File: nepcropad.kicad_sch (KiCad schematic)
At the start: 34 parts, among them SW1 SW_Push, U1 ATmega32U4-A, Y1 16MHz

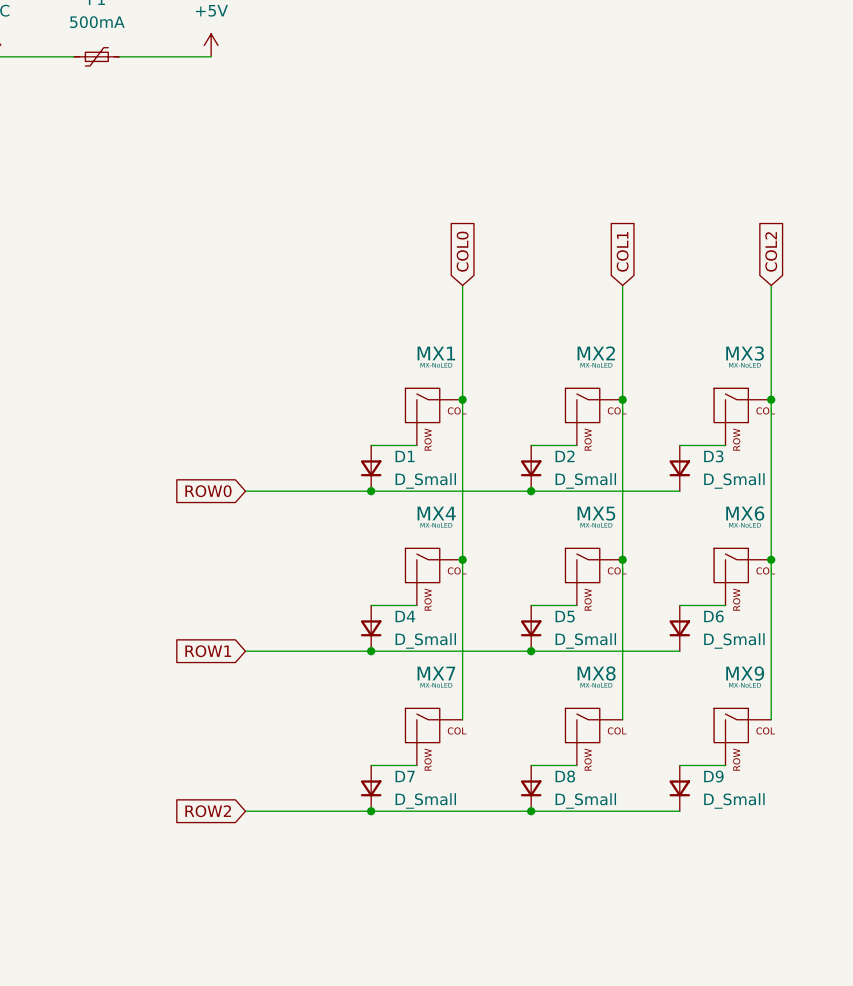
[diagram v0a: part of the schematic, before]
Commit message: PCB Layout
did the pcb layout
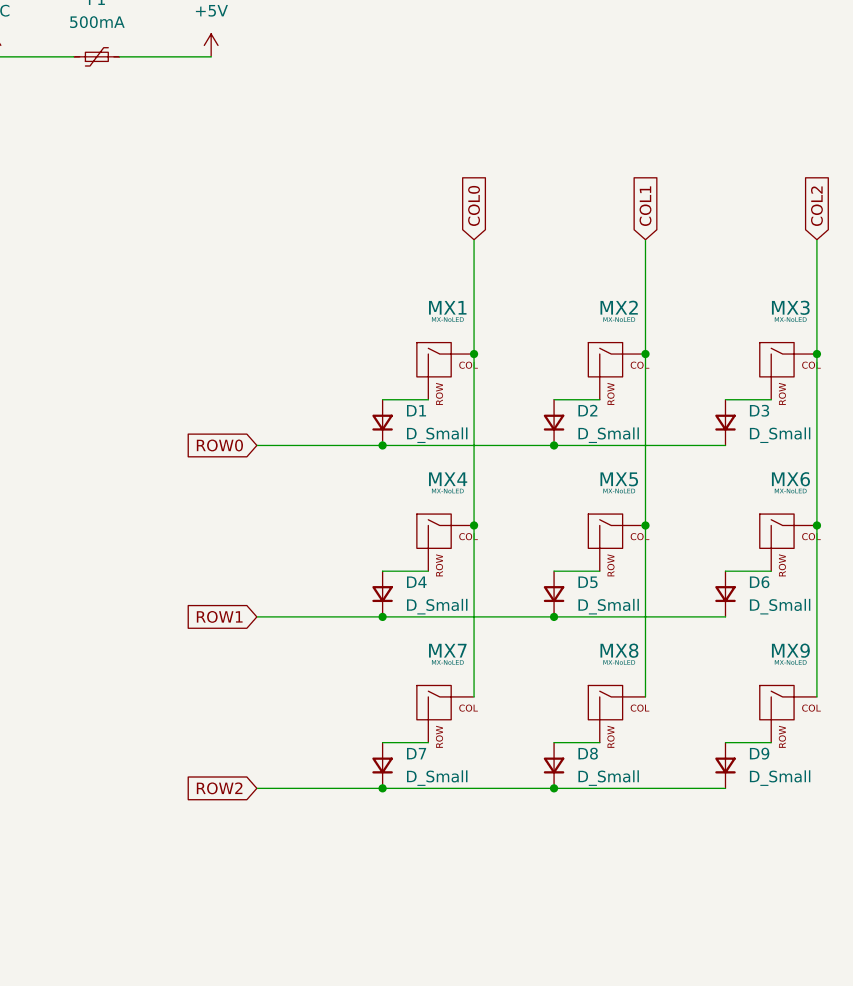
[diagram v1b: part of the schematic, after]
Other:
- moved on the sheet: D1, D2, D3, D4, D5, D6, D7, D8, D9, MX1, MX2, MX3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

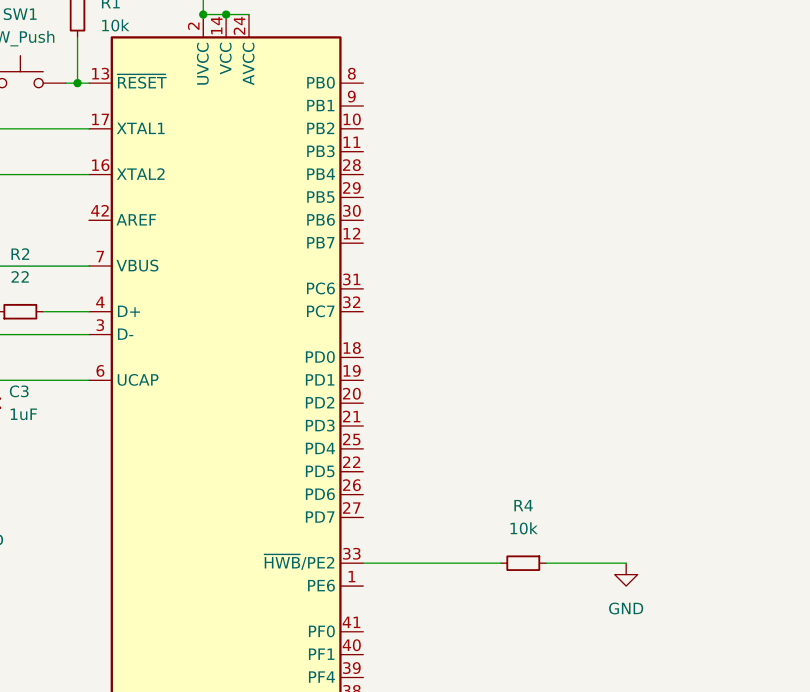
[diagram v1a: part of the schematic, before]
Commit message: Finished routing
I think atleast.
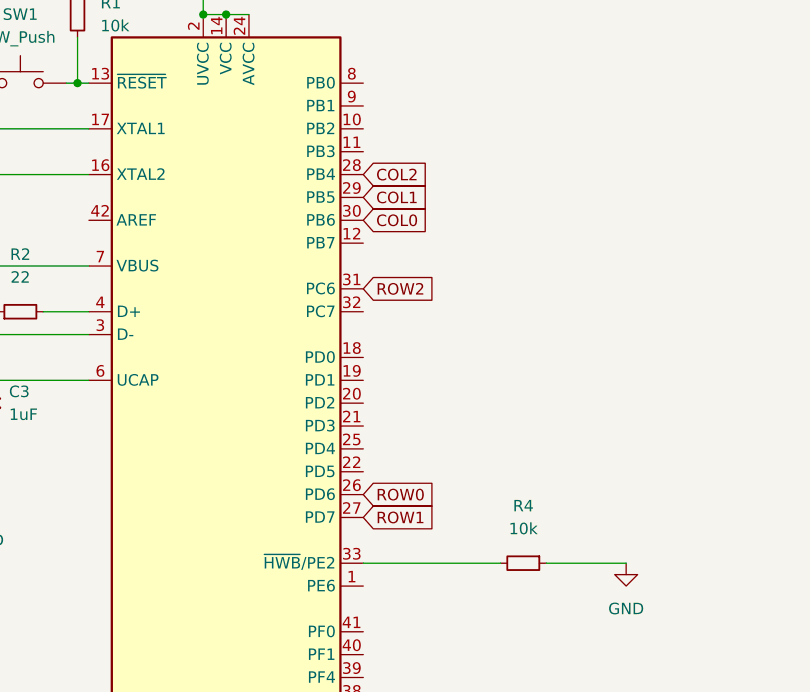
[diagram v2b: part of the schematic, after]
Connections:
- net COL0: now also U1.30 (PB6)
- net COL1: now also U1.29 (PB5)
- net COL2: now also U1.28 (PB4)
- net ROW0: now also U1.26 (PD6)
- net ROW1: now also U1.27 (PD7)
- net ROW2: now also U1.31 (PC6)
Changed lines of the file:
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@@
+    )
+  )
+  (global_label "ROW1" (shape input) (at 104.14 119.38 0) (fields_autoplaced)
+    (effects (font (size 1.27 1.27)) (justify left))
+    (property "Intersheet References" "${INTERSHEET_REFS}" (id 0) (at 111.8145 119.3006 0)
+      (effects (font (size 1.27 1.27)) (justify left) hide)
+    )
+  )
+  (global_label "ROW2" (shape input) (at 104.14 93.98 0) (fields_autoplaced)
+    (effects (font (size 1.27 1.27)) (justify left))
+    (property "Intersheet References" "${INTERSHEET_REFS}" (id 0) (at 111.8145 93.9006 0)
+      (effects (font (size 1.27 1.27)) (justify left) hide)
     )
   )
@@
     (effects (font (size 1.27 1.27)) (justify left))
     (property "Intersheet References" "${INTERSHEET_REFS}" (id 0) (at 136.0655 35.6394 0)
+      (effects (font (size 1.27 1.27)) (justify left) hide)
+    )
+  )
+  (global_label "ROW0" (shape input) (at 104.14 116.84 0) (fields_autoplaced)
+    (effects (font (size 1.27 1.27)) (justify left))
+    (property "Intersheet References" "${INTERSHEET_REFS}" (id 0) (at 111.8145 116.7606 0)
       (effects (font (size 1.27 1.27)) (justify left) hide)
     )
@@
     )
   )
+  (global_label "COL2" (shape input) (at 104.14 81.28 0) (fields_autoplaced)
+    (effects (font (size 1.27 1.27)) (justify left))
+    (property "Intersheet References" "${INTERSHEET_REFS}" (id 0) (at 111.3912 81.2006 0)
+      (effects (font (size 1.27 1.27)) (justify left) hide)
+    )
+  )
+  (global_label "COL1" (shape input) (at 104.14 83.82 0) (fields_autoplaced)
+    (effects (font (size 1.27 1.27)) (justify left))
+    (property "Intersheet References" "${INTERSHEET_REFS}" (id 0) (at 111.3912 83.7406 0)
+      (effects (font (size 1.27 1.27)) (justify left) hide)
+    )
+  )
   (global_label "ROW2" (shape input) (at 166.37 114.3 180) (fields_autoplaced)
     (effects (font (size 1.27 1.27)) (justify right))
@@
       (effects (font (size 1.27 1.27)) (justify left) hide)
     )
+  )
+  (global_label "COL0" (shape input) (at 104.14 86.36 0) (fields_autoplaced)
+    (effects (font (size 1.27 1.27)) (justify left))
+    (property "Intersheet References" "${INTERSHEET_REFS}" (id 0) (at 111.3912 86.2806 0)
+      (effects (font (size 1.27 1.27)) (justify left) hide)
+    )

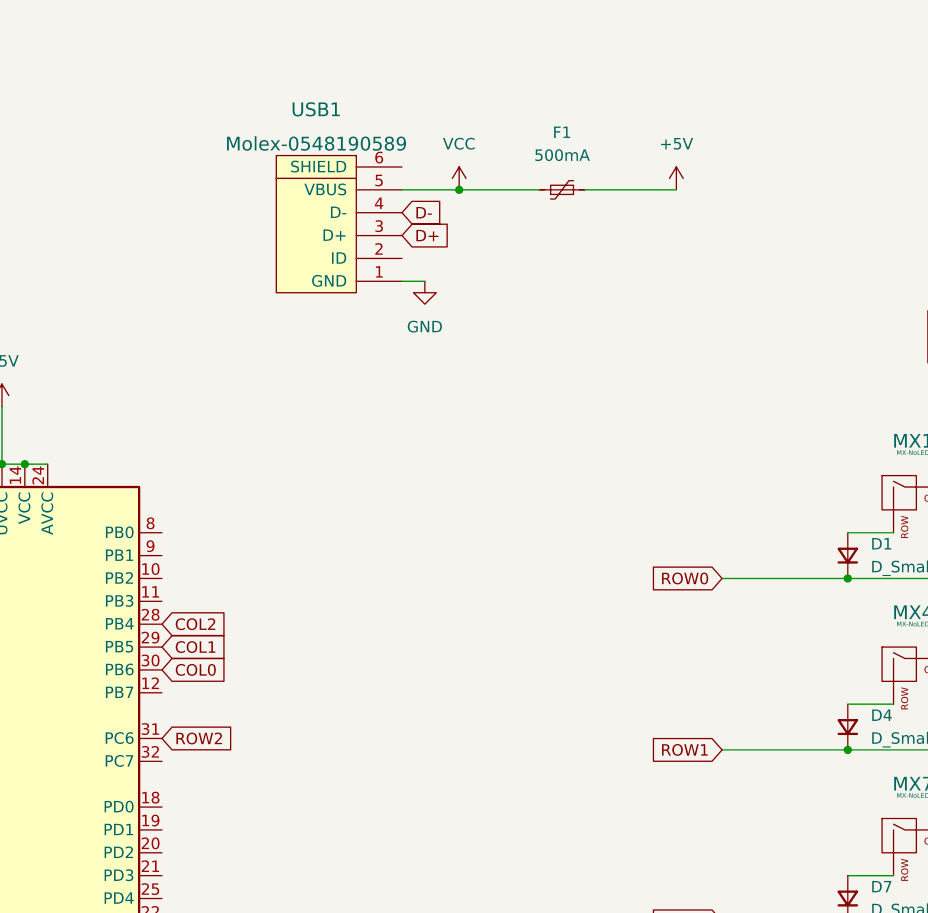
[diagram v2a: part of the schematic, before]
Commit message: minimize pcb
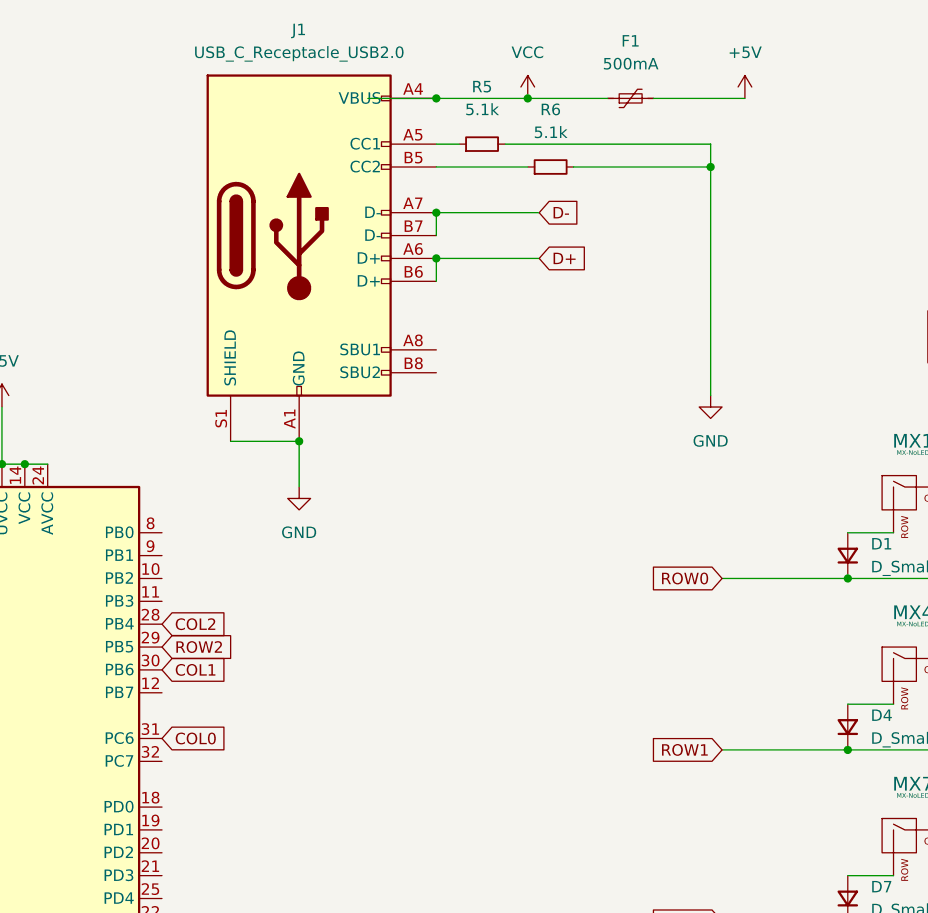
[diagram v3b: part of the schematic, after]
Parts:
- removed USB1: Molex-0548190589, random-keyboard-parts:Molex-0548190589, symbol random-keyboard-parts:Molex-0548190589
- added J1: USB_C_Receptacle_USB2.0, usbc:USB_C_GCT_USB4085, symbol symbols:USB_C_Receptacle_USB2.0
- added R5, R6: 5.1k, resistor:R_0805_2012Metric, symbol device:R_Small
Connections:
- net COL0: now also U1.31 (PC6); no longer U1.30 (PB6)
- net COL1: now also U1.30 (PB6); no longer U1.29 (PB5)
- net D+: now also J1.A6 (D+), J1.B6 (D+)
- net D-: now also J1.A7 (D-), J1.B7 (D-)
- net GND: now also J1.A1 (GND), J1.A12 (GND), J1.B1 (GND), J1.B12 (GND), J1.S1 (SHIELD), R5.2, R6.2
- net ROW2: now also U1.29 (PB5); no longer U1.31 (PC6)
- net VCC: now also J1.A4 (VBUS), J1.A9 (VBUS), J1.B4 (VBUS), J1.B9 (VBUS)
- new net: J1.A5 (CC1), R5.1
- new net: J1.B5 (CC2), R6.1
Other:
- moved on the sheet: F1
